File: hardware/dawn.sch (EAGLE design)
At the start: 50 parts, among them IC1 LM393N, IC2 AT90S2313P, IC3 DS1307, Q1 IRFU9024N, Q2 4Mhz, Q3 32.768kHz, T1 BC457B, T2 BC557B

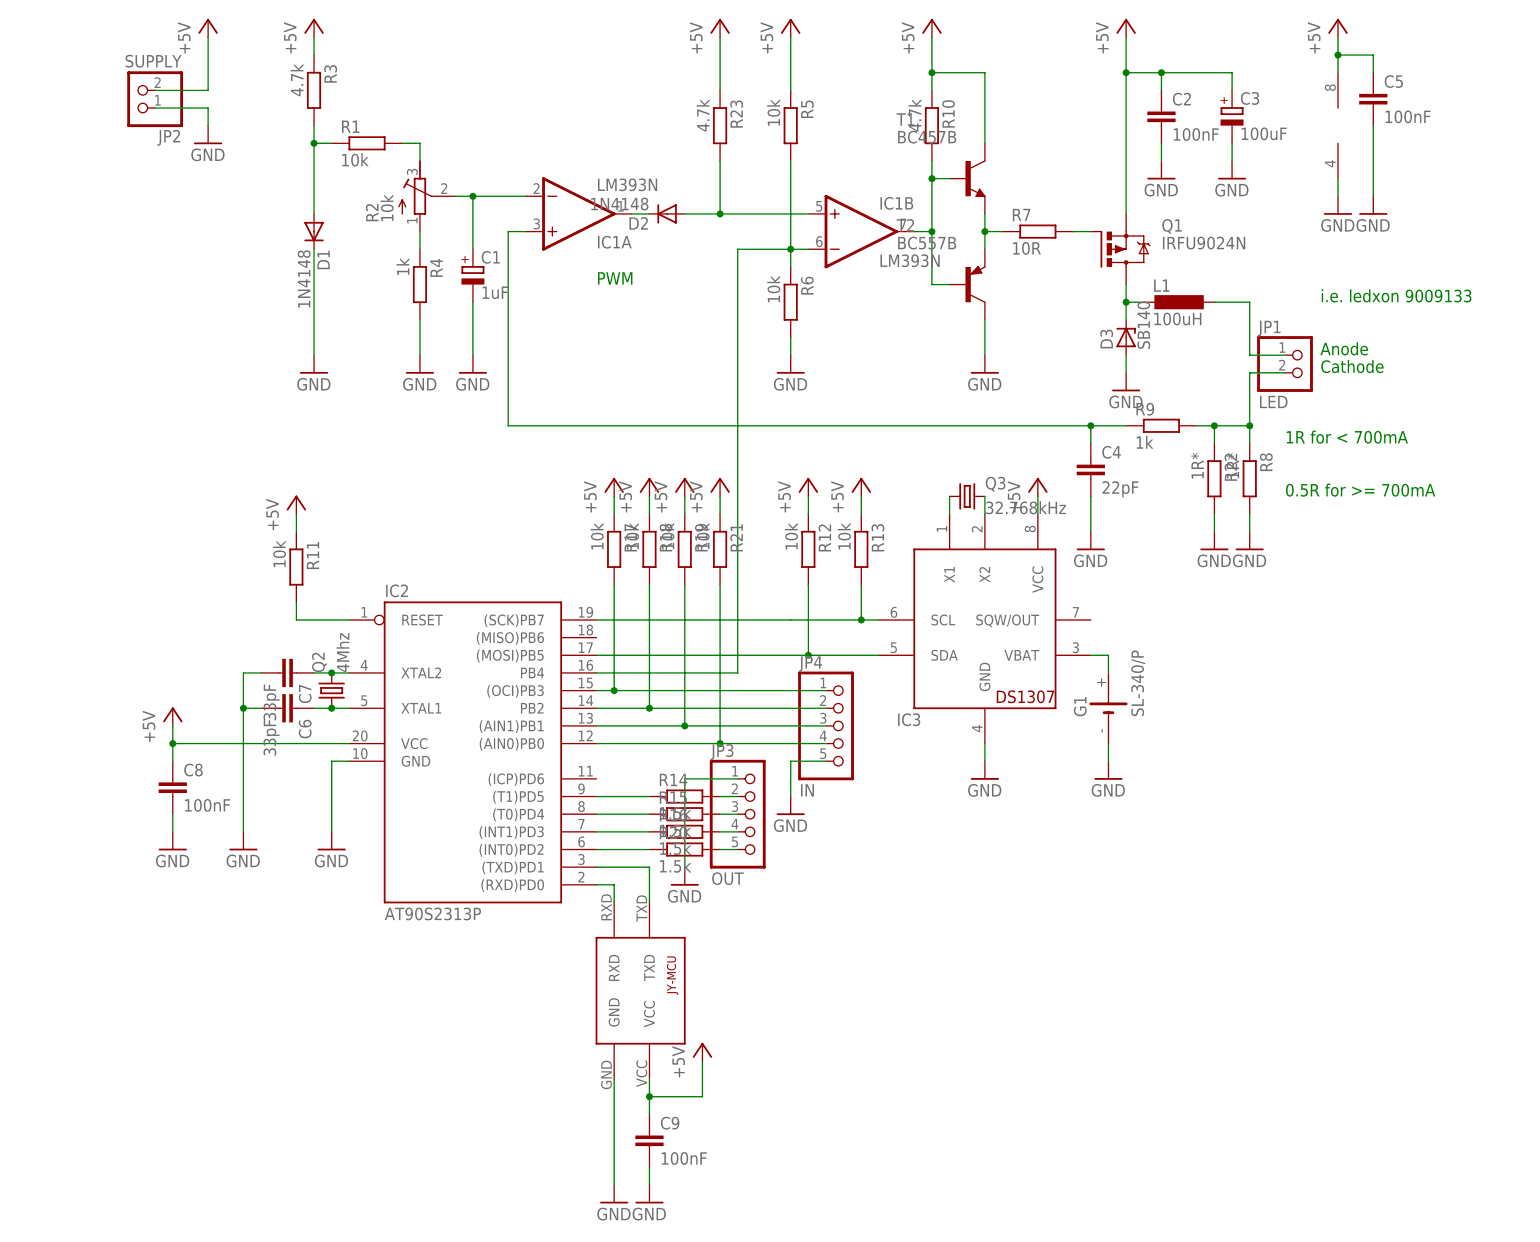
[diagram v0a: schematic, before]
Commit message: Fixed schematic & board.
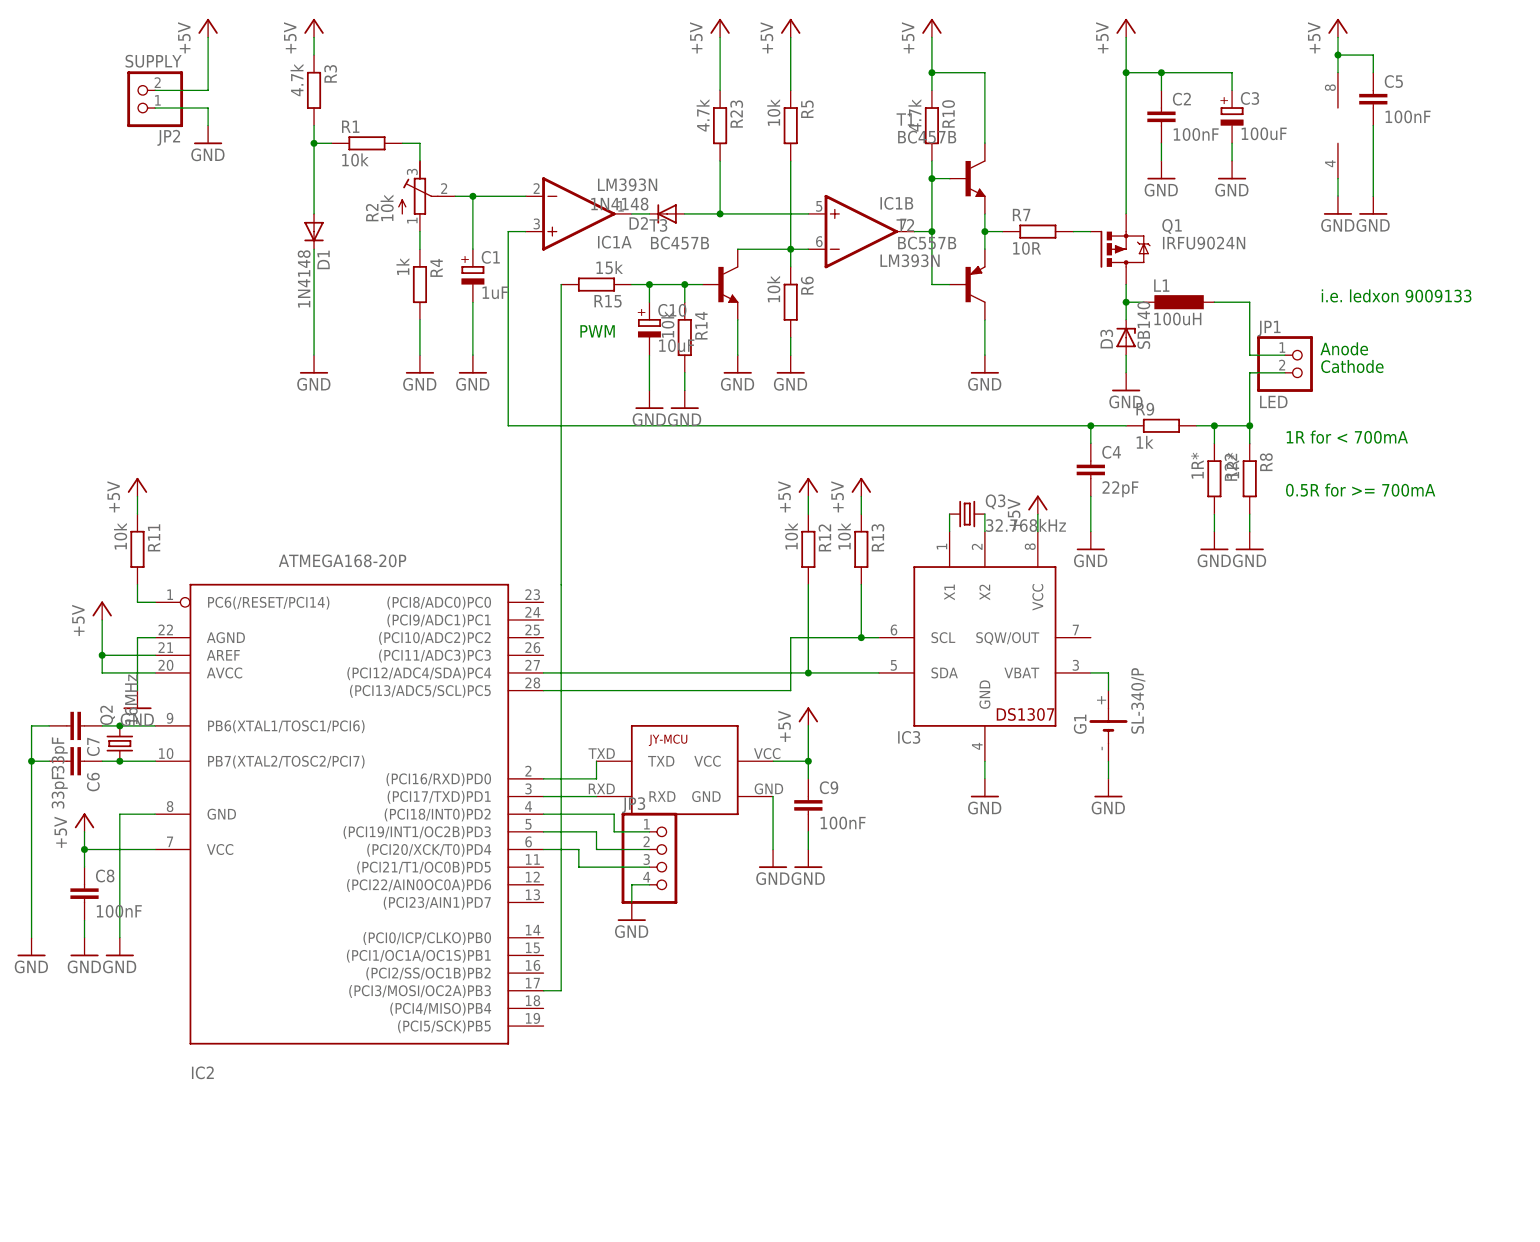
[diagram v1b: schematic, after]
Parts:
- removed JP4: IN, pinhead:PINHD-1X5
- removed R16, R20: 1.5k, rcl:R-EU_0204/5
- removed R17: 10k, rcl:R-EU_0207/10
- removed R18: 10k, rcl:R-EU_0207/12
- removed R19: 10k, rcl:R-EU_0207/15
- removed R21: 10k, rcl:R-EU_0204/5
- added C10: 10uF, rcl:CPOL-EUE2,5-6E
- added T3: BC457B, transistor:-NPN-TO92-EBC
- C6: device rcl:C-EU025-025X050 -> rcl:C-EU050-025X075
- C8: device rcl:C-EU050-025X075 -> rcl:C-EU025-025X050
- IC2: value AT90S2313P -> ATMEGA168-20P; device atmel:AT90S2313P -> adafruit:ATMEGA168-20P
- JP3: value OUT -> (none); device pinhead:PINHD-1X5 -> pinhead:PINHD-1X4
- Q2: value 4Mhz -> 16MHz; device adafruit:CRYSTALHC18U-V -> crystal:CRYSTALHC49S
- R11: device rcl:R-EU_0207/10 -> rcl:R-EU_0204/2V
- R12: device rcl:R-EU_0204/7 -> rcl:R-EU_0204/5
- R14: value 1.5k -> 10k; device rcl:R-EU_0204/5 -> rcl:R-EU_0204/2V
- R15: value 1.5k -> 15k; device rcl:R-EU_0204/5 -> rcl:R-EU_0207/10
- R6: device rcl:R-EU_0207/12 -> rcl:R-EU_0207/10
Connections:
- removed net N$29: IC2.(T0)PD4, R15.1
- removed net N$31: IC2.(OCI)PB3, JP4.1, R17.2
- removed net N$32: IC2.PB2, JP4.2, R18.2
- removed net N$33: IC2.(AIN1)PB1, JP4.3, R19.2
- removed net N$34: JP3.5, R20.2
- removed net N$35: IC2.(INT0)PD2, R20.1
- removed net N$36: IC2.(AIN0)PB0, JP4.4, R21.2
- net +5V: now also IC2.AREF, IC2.AVCC; no longer R17.1, R18.1, R19.1, R21.1
- net GND: now also C10.-, IC2.AGND, JP3.4, R14.2, T3.E; no longer JP3.1, JP4.5
- net N$12: now also IC2.(PCI17/TXD)PD1, U$1.RXD; no longer C7.1, IC2.XTAL2, Q2.2
- net N$18: now also IC2.PB7(XTAL2/TOSC2/PCI7); no longer IC2.XTAL1
- net N$19: now also IC2.(PCI13/ADC5/SCL)PC5; no longer IC2.(SCK)PB7
- net N$20: now also IC2.PC6(/RESET/PCI14); no longer IC2.RESET
- net N$21: now also IC2.(PCI12/ADC4/SDA)PC4; no longer IC2.(MOSI)PB5
- net N$23: now also IC2.(PCI16/RXD)PD0; no longer IC2.(TXD)PD1
- net N$24: now also IC2.(PCI18/INT0)PD2, JP3.1; no longer IC2.(RXD)PD0, U$1.RXD
- net N$25: now also IC2.(PCI3/MOSI/OC2A)PB3, R15.2; no longer JP3.2, R14.2
- net N$26: now also C10.+, R14.1, R15.1, T3.B; no longer JP3.3, R15.2
- net N$27: now also IC2.(PCI19/INT1/OC2B)PD3, JP3.2; no longer JP3.4, R16.2
- net N$28: now also IC2.(PCI20/XCK/T0)PD4, JP3.3; no longer IC2.(INT1)PD3, R16.1
- net N$30: now also C7.1, IC2.PB6(XTAL1/TOSC1/PCI6), Q2.2; no longer IC2.(T1)PD5, R14.1
- net N$9: now also T3.C; no longer IC2.PB4
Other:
- moved on the sheet: C6, C7, C8, C9, G1, IC3, Q2, Q3, R11, R14, R15
